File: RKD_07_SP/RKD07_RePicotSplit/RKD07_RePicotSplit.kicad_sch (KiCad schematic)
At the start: 20 parts, among them J1 Conn_01x24, J2 Conn_01x06, J3 Conn_01x06, J4 Conn_01x12, J51 Conn_01x06, J52 Qwiic_RA, J53 6P6C, J54 Conn_01x02_Socket, SW25 RotaryEncoder_Switch, SW31 SW_Push, SW53 SW_Push, SW55 SW_Push, U1 Pico

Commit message: update
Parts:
- added C201, C203, C206, C207: 0.1uF X7R, Capacitor_SMD:C_0805_2012Metric_Pad1.18x1.45mm_HandSolder, symbol Device:C_Small
- added C202: 1uF, Capacitor_SMD:C_0805_2012Metric_Pad1.18x1.45mm_HandSolder, symbol Device:C_Small
- added C204, C208: 0.01uF X7R, Capacitor_SMD:C_0805_2012Metric_Pad1.18x1.45mm_HandSolder, symbol Device:C_Small
- added C205: 10uF X7R, Capacitor_SMD:C_0805_2012Metric_Pad1.18x1.45mm_HandSolder, symbol Device:C_Small
- added C209: 3.3uF/16V, Capacitor_SMD:C_0805_2012Metric_Pad1.18x1.45mm_HandSolder, symbol Device:C_Small
- added J101: Conn_01x24, Connector_FFC-FPC:Hirose_FH12-24S-0.5SH_1x24-1MP_P0.50mm_Horizontal, symbol Connector_Generic:Conn_01x24
- added J104, J5: Conn_01x06, DreaM117er-keebLibrary:Hirose_FH12-6S-0.5SH_1x06-1MP_P0.50mm_Horizontal, symbol Connector_Generic:Conn_01x06
- added J105: Conn_01x12, DreaM117er-keebLibrary:Hirose_FH12-12S-0.5SH_1x12-1MP_P0.50mm_Horizontal, symbol Connector_Generic:Conn_01x12
- added J151: Conn_01x06, Connector_PinHeader_2.54mm:PinHeader_1x08_P2.54mm_Vertical, symbol Connector_Generic:Conn_01x08
- added J153: 6P6C, Connector_RJ:RJ12_Amphenol_54601-x06_Horizontal, symbol Connector:6P6C
- added J155: Conn_01x08, Connector_PinHeader_2.54mm:PinHeader_1x08_P2.54mm_Vertical, symbol Connector_Generic:Conn_01x08
- added J2, J201: Conn_01x06, Connector_FFC-FPC:Hirose_FH12-6S-0.5SH_1x06-1MP_P0.50mm_Horizontal, symbol Connector_Generic:Conn_01x06
- added J251, J253, J254, J54: Conn_01x02_Socket, Connector_PinHeader_2.54mm:PinHeader_1x02_P2.54mm_Vertical, symbol Connector_Generic:Conn_01x02
- added J252: Conn_01x06, Connector_PinHeader_2.54mm:PinHeader_1x06_P2.54mm_Vertical, symbol Connector_Generic:Conn_01x06
- added OL101: OLED, BrownSugar_KBD:OLED_center_display, symbol BrownSugar_KBD:OLED
- added R201: 10k, Resistor_SMD:R_0805_2012Metric_Pad1.20x1.40mm_HandSolder, symbol Device:R
- added U101: Pico, Rikkodo_FootPrint:rkd_RPi_Pico_TH_NODBG, symbol RPi_Pico:Pico
- added U201: TLV70019DDCR, Package_TO_SOT_SMD:SOT-23-5_HandSoldering, symbol Regulator_Linear:TLV70019_SOT23-5
- added U202: PMW3610DM-SUDU, Rikkodo_FootPrint:PMW3610DM-SUDU, symbol seiboku-symbols:PMW3610-SUDU
- renumbered J2 to J102, J54 to J154
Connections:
- net 3V3_R: now also J2.6 (Pin_6); no longer J102.6 (Pin_6)
- net COL10_R: now also J5.3 (Pin_3)
- net COL6_R: now also J5.1 (Pin_1)
- net COL7_R: now also J5.2 (Pin_2)
- net GND_R: now also J2.1 (Pin_1), J2.5 (Pin_5), J5.6 (Pin_6); no longer J102.1 (Pin_1), J102.5 (Pin_5)
- net GP00_MISO_R: now also J2.4 (Pin_4); no longer J102.4 (Pin_4)
- net GP02_SCLK_R: now also J2.3 (Pin_3); no longer J102.3 (Pin_3)
- net GP03_MOSI_R: now also J2.2 (Pin_2); no longer J102.2 (Pin_2)
- net GP04_RE_A_R: now also J5.5 (Pin_5), J54.1 (Pin_1); no longer J154.1 (Pin_1)
- net GP07_RE_B_R: now also J5.4 (Pin_4), J54.2 (Pin_2); no longer J154.2 (Pin_2)
- new net: C204.1, U202.1 (+VCSEL), U202.10 (PASS_T)
- new net: R201.1, U202.7 (NRESET)
- new net: C207.1, U202.13 (CN)
- new net: C207.2, U202.12 (CP)
- new net: C205.1, C208.1, U202.9 (VCP)
- new net: U202.15 (XYLASER), U202.16 (-VCSEL)
- new net 1V9_E: C202.1, C206.1, C209.1, U201.5 (OUT), U202.14 (VDD)
- new net 3V3_E: C201.1, C203.1, J201.1 (Pin_1), J252.6 (Pin_6), R201.2, U201.1 (IN), U201.3 (EN), U202.6 (VDDIO)
- new net 3V3_L: J101.3 (Pin_3), J102.6 (Pin_6), J151.8 (Pin_8), J155.7 (Pin_7), OL101.3 (VCC), U101.36 (3V3)
- new net COL0_L: J101.15 (Pin_15), U101.7 (GPIO5)
- new net COL10_L: J101.8 (Pin_8), J104.3 (Pin_3), J155.4 (Pin_4), U101.29 (GPIO22)
- new net COL11_L: J101.7 (Pin_7), J105.9 (Pin_9), J155.5 (Pin_5), U101.31 (GPIO26_ADC0)
- new net COL12_L: J101.6 (Pin_6), J105.10 (Pin_10), J155.6 (Pin_6), U101.32 (GPIO27_ADC1)
- new net COL13_GP01_NCS_L: J101.5 (Pin_5), J104.2 (Pin_2), J151.4 (Pin_4), U101.2 (GPIO1)
- new net COL1_L: J101.16 (Pin_16), U101.9 (GPIO6)
- new net COL2_L: J101.17 (Pin_17), U101.11 (GPIO8)
- new net COL3_L: J101.18 (Pin_18), U101.12 (GPIO9)
- new net COL4_L: J101.19 (Pin_19), U101.14 (GPIO10)
- new net COL5_L: J101.20 (Pin_20), U101.15 (GPIO11)
- new net COL6_GP16_L: J101.12 (Pin_12), J105.11 (Pin_11), J153.3, U101.21 (GPIO16)
- new net COL7_GP17_L: J101.11 (Pin_11), J105.12 (Pin_12), J153.4, U101.22 (GPIO17)
- new net COL8_L: J101.10 (Pin_10), J105.7 (Pin_7), J155.2 (Pin_2), U101.26 (GPIO20)
- new net COL9_L: J101.9 (Pin_9), J105.8 (Pin_8), J155.3 (Pin_3), U101.27 (GPIO21)
- new net GND_E: C201.2, C202.2, C203.2, C204.2, C205.2, C206.2, C208.2, C209.2, J201.6 (Pin_6), J251.1 (Pin_1), J252.1 (Pin_1), U201.2 (GND), U202.11 (GND)
- new net GND_L: J101.1 (Pin_1), J102.1 (Pin_1), J102.5 (Pin_5), J104.6 (Pin_6), J105.1 (Pin_1), J151.1 (Pin_1), J151.2 (Pin_2), J151.3 (Pin_3), J153.2, J155.1 (Pin_1), OL101.4 (GND), U101.13 (GND), U101.18 (GND), U101.23 (GND), U101.28 (GND), U101.3 (GND), U101.38 (GND), U101.8 (GND)
- new net GP00_MISO_E: J201.3 (Pin_3), J252.4 (Pin_4), U202.2 (SDIO)
- new net GP00_MISO_L: J102.4 (Pin_4), J151.5 (Pin_5), U101.1 (GPIO0)
- new net GP02_SCLK_E: J201.4 (Pin_4), J252.3 (Pin_3), U202.3 (SCLK)
- new net GP02_SCLK_L: J102.3 (Pin_3), J151.6 (Pin_6), U101.4 (GPIO2)
- new net GP03_MOSI_E: J201.5 (Pin_5), J252.2 (Pin_2), U202.8 (MOTION)
- new net GP03_MOSI_L: J102.2 (Pin_2), J151.7 (Pin_7), U101.5 (GPIO3)
- new net GP04_E: J253.1 (Pin_1), J254.2 (Pin_2)
- new net GP04_L: J104.5 (Pin_5), J154.1 (Pin_1), U101.6 (GPIO4)
- new net GP07_E: J253.2 (Pin_2), J254.1 (Pin_1)
- new net GP07_L: J104.4 (Pin_4), J154.2 (Pin_2), U101.10 (GPIO7)
- new net NCS_E: J201.2 (Pin_2), J251.2 (Pin_2), J252.5 (Pin_5), U202.5 (NCS)
- new net ROW0_L: J101.4 (Pin_4), J105.2 (Pin_2), U101.34 (GPIO28_ADC2)
- new net ROW1_L: J101.21 (Pin_21), J105.6 (Pin_6), U101.16 (GPIO12)
- new net ROW2_L: J101.22 (Pin_22), J105.5 (Pin_5), U101.17 (GPIO13)
- new net ROW3_L: J101.23 (Pin_23), J105.4 (Pin_4), U101.19 (GPIO14)
- new net ROW4_L: J101.24 (Pin_24), J105.3 (Pin_3), U101.20 (GPIO15)
- new net SCL/TX_L: J101.13 (Pin_13), OL101.2 (SCL), U101.25 (GPIO19)
- new net SDA/SCK_L: J101.14 (Pin_14), OL101.1 (SDA), U101.24 (GPIO18)
- new net VCC_L: J101.2 (Pin_2), J153.5, J155.8 (Pin_8), U101.39 (VSYS)
- no-connect marks 12 -> 23
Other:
- note added: "3V3 NCS SDIO SCLK MOTION GND"
- note added: "GND GP01_NCS GP00_MISO GP02_SCLK GP03_MOSI"
- note added: "GND MOTION SCLK SDIO NCS 3V3"
- note added: "Receive"
- moved on the sheet: J102, J154

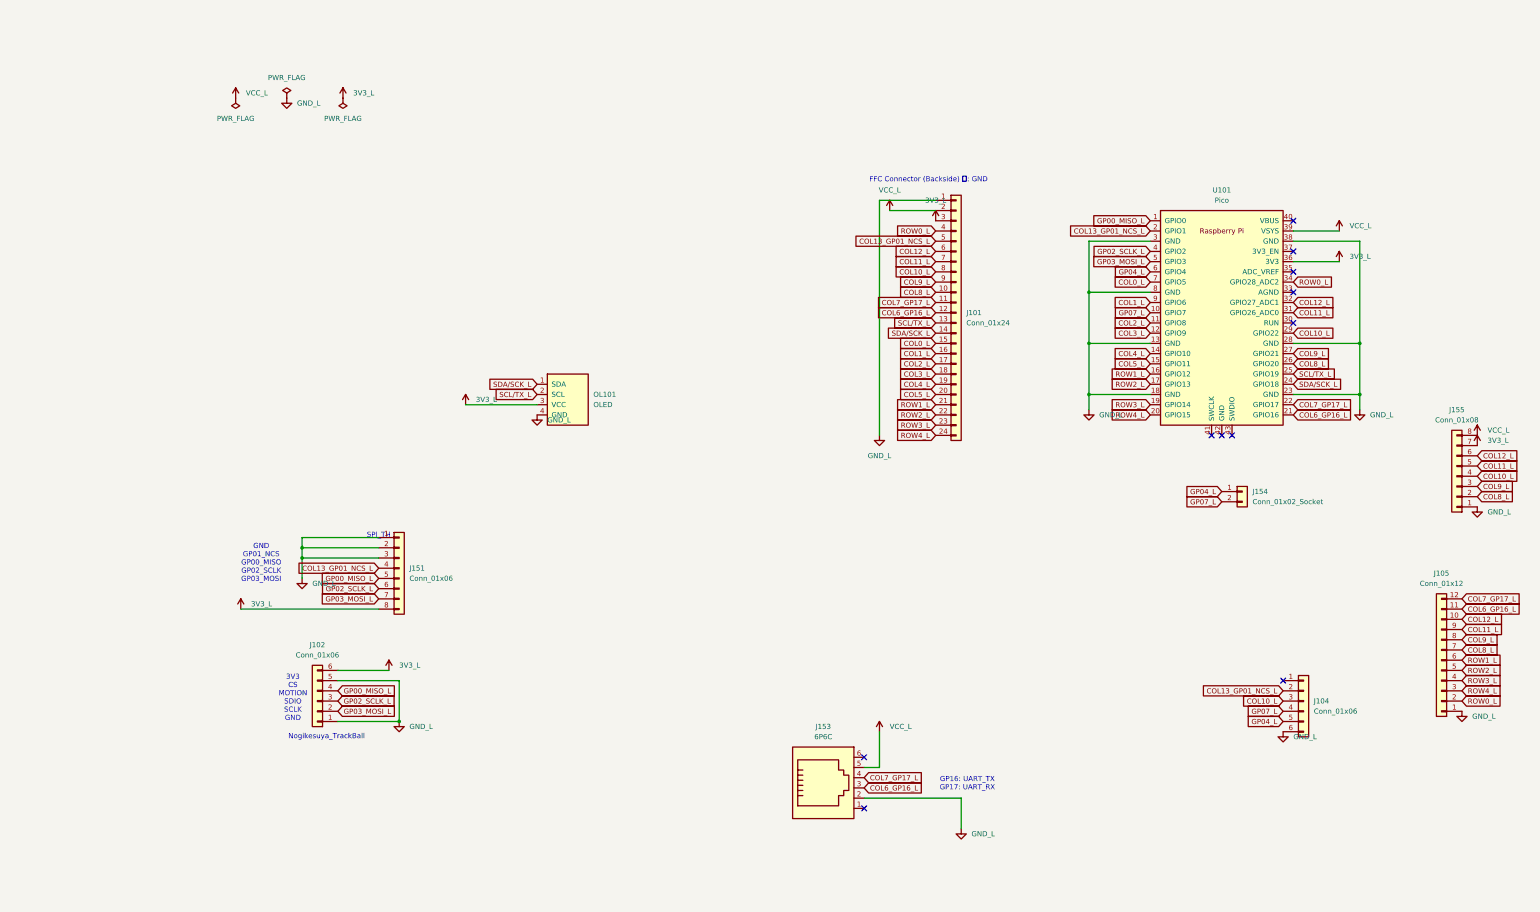
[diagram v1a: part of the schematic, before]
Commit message: modify
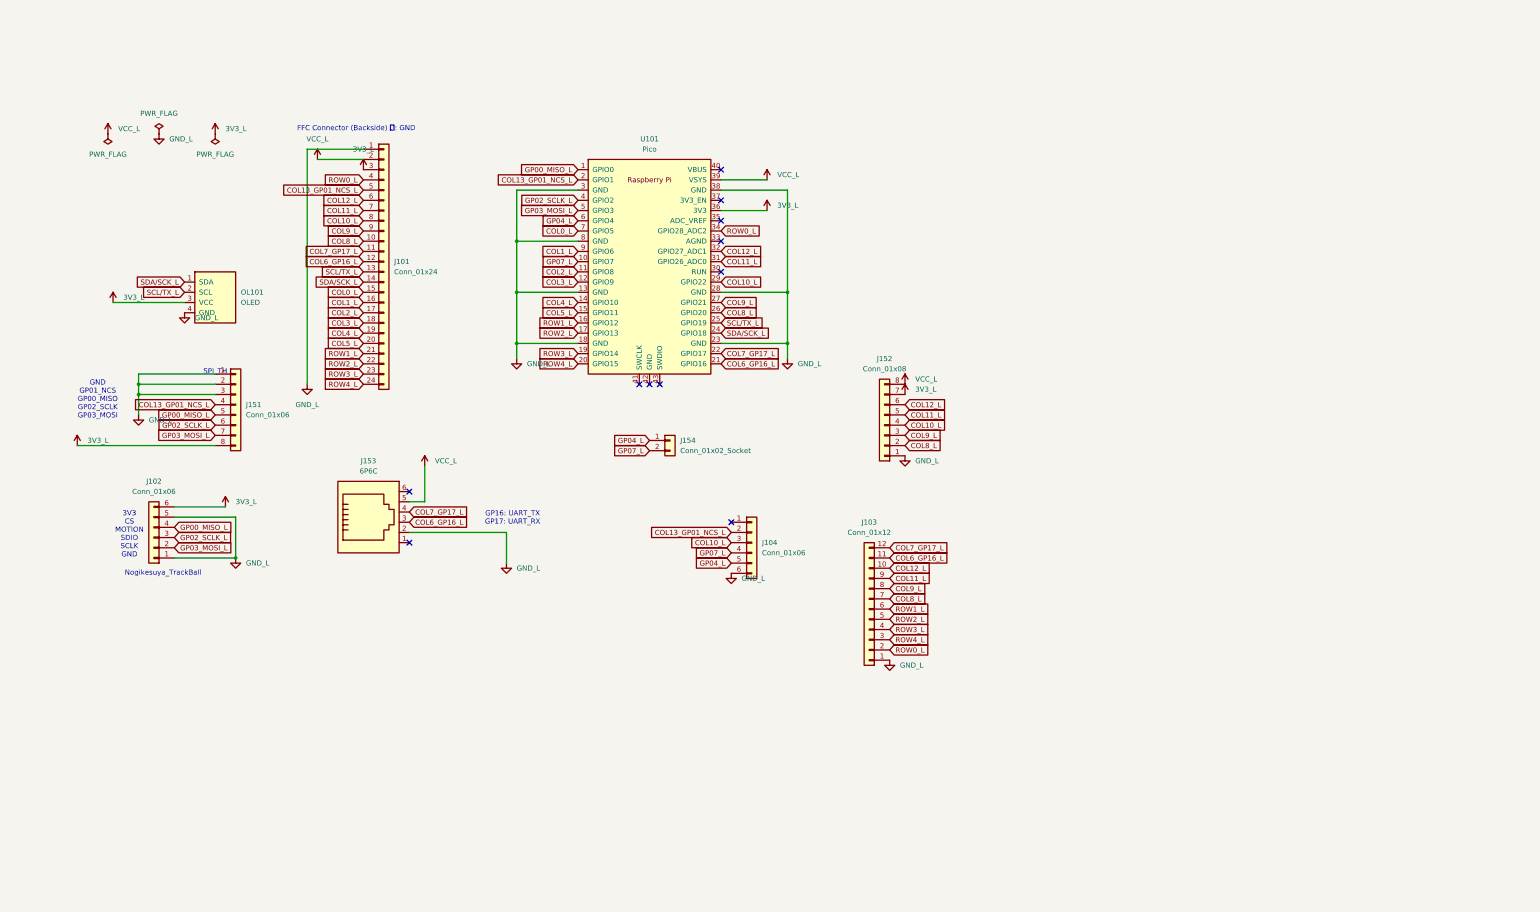
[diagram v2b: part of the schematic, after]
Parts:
- renumbered J105 to J103, J155 to J152
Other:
- moved on the sheet: J101, J102, J103, J104, J151, J152, J153, J154, OL101, U101
